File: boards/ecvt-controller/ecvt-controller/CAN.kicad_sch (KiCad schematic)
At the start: 12 parts, among them SW1 SW_SPST, SW2 SW_SPST, U1 TJA1051T-3

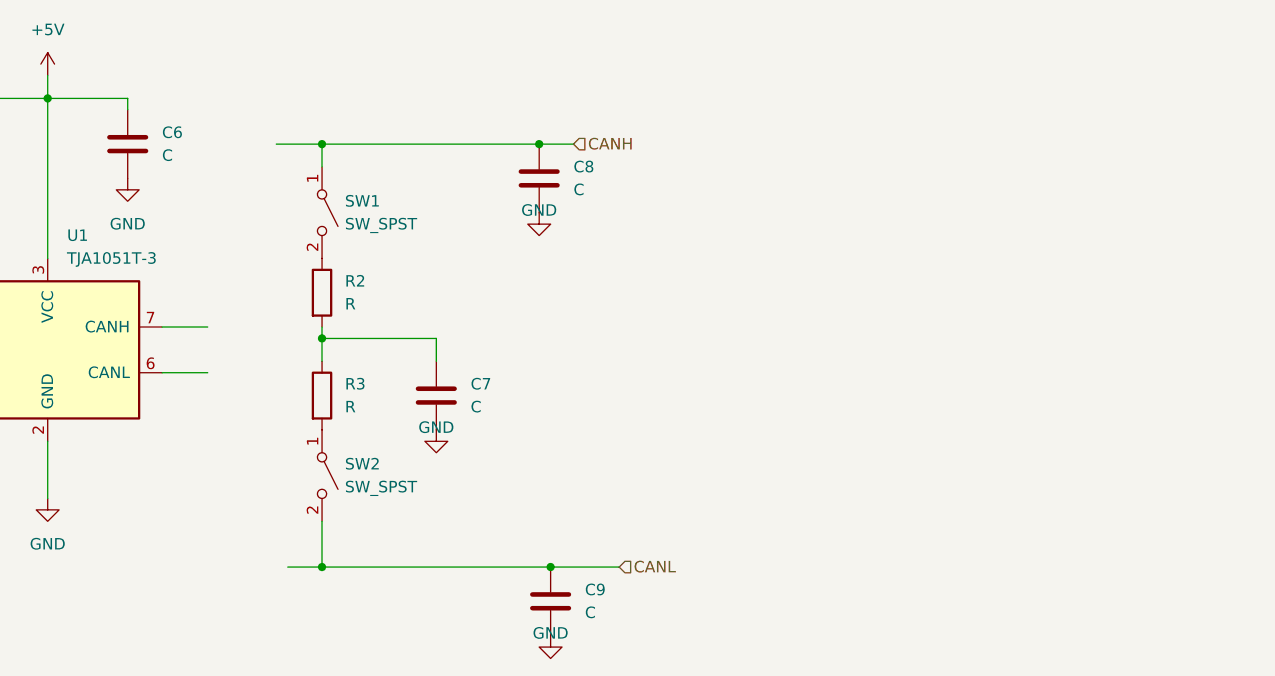
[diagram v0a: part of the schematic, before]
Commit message: CAN
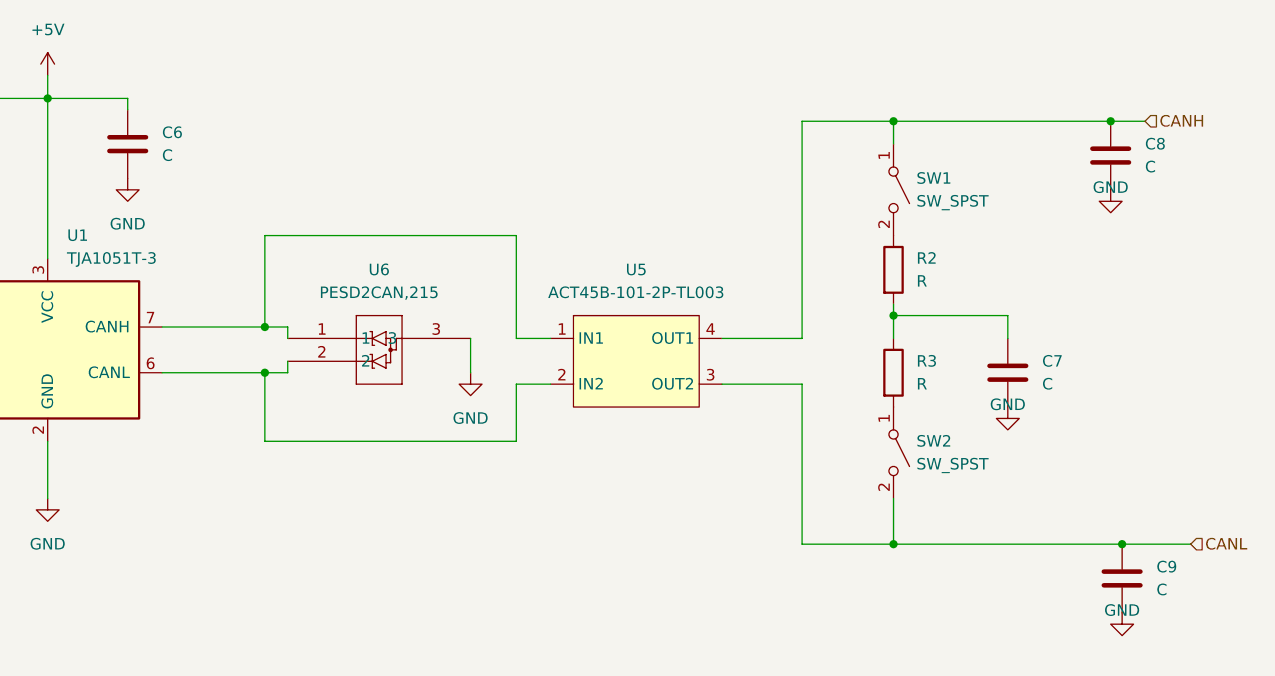
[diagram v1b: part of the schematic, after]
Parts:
- added U5: ACT45B-101-2P-TL003, baja_footprint_library:ACT45B-101-2P-TL003, symbol baja_symbol_library:ACT45B-101-2P-TL003
- added U6: PESD2CAN,215, Package_TO_SOT_SMD:SOT-23, symbol baja_symbol_library:ESD3V3AP-TP
- SW1, SW2: footprint (none) -> Button_Switch_THT:SW_DIP_SPSTx01_Slide_9.78x4.72mm_W7.62mm_P2.54mm
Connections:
- net CANH: now also U5.4 (OUT1)
- net CANL: now also U5.3 (OUT2)
- net GND: now also U6.3
- net at U1.6 (CANL): now also U5.2 (IN2), U6.2
- net at U1.7 (CANH): now also U5.1 (IN1), U6.1
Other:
- moved on the sheet: C7, C8, C9, R2, R3, SW1, SW2

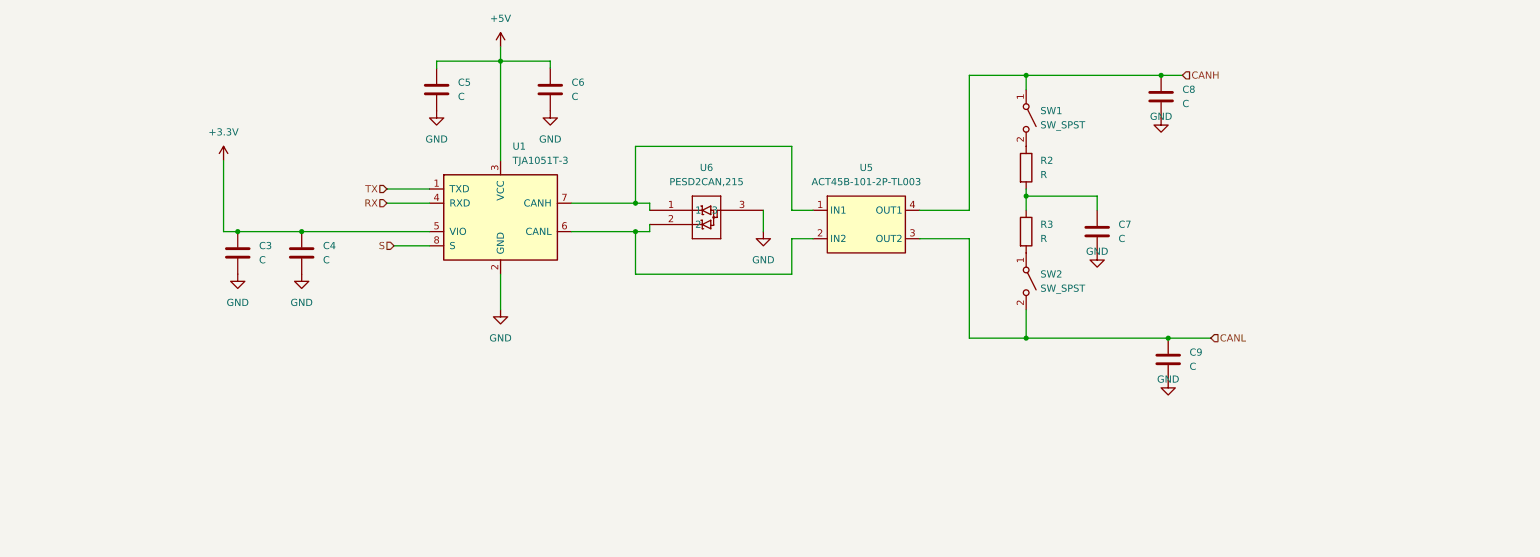
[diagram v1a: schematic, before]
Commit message: CAN actually done
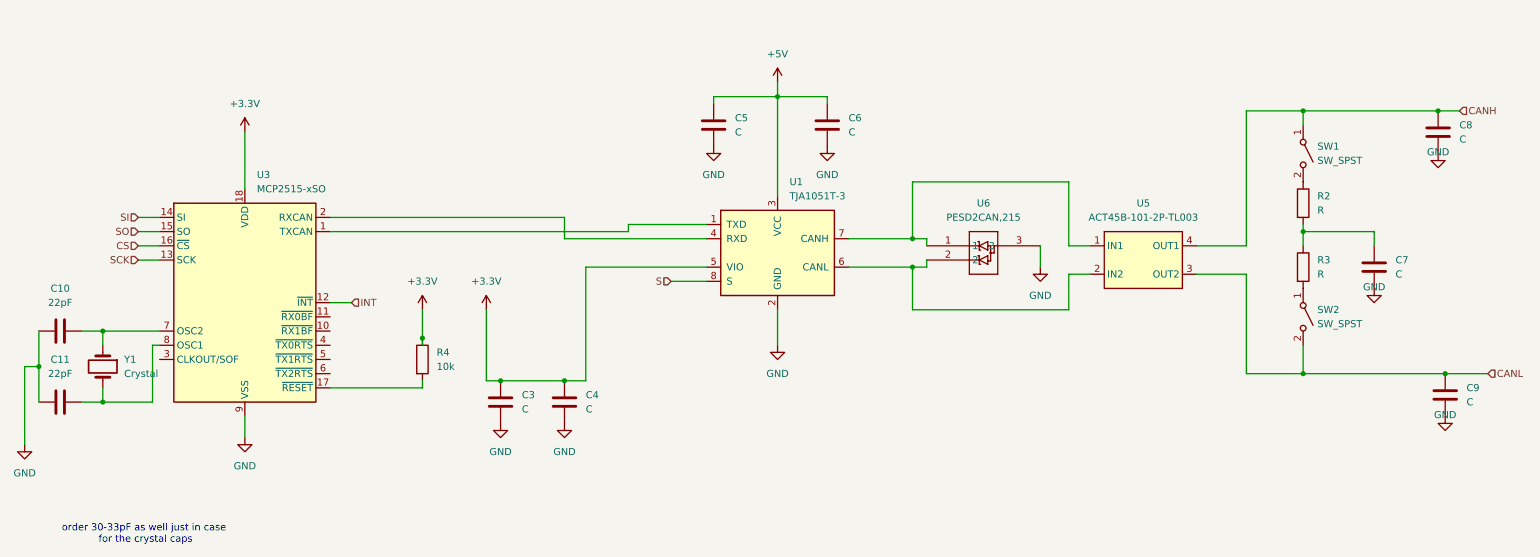
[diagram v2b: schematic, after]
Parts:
- added C10, C11: 22pF, symbol Device:C
- added R4: 10k, symbol Device:R
- added U3: MCP2515-xSO, Package_SO:SOIC-18W_7.5x11.6mm_P1.27mm, symbol Interface_CAN_LIN:MCP2515-xSO
- added Y1: Crystal, Crystal:Crystal_SMD_5032-2Pin_5.0x3.2mm_HandSoldering, symbol Device:Crystal
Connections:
- net +3.3V: now also R4.1, U3.18 (VDD)
- net GND: now also C10.1, C11.1, U3.9 (VSS)
- net RX: no longer names the net of U1.4 (RXD)
- net RX: now also U3.2 (RXCAN)
- net TX: no longer names the net of U1.1 (TXD)
- net TX: now also U3.1 (TXCAN)
- new net: R4.2, U3.17 (~{RESET})
- new net: C10.2, U3.7 (OSC2), Y1.1
- new net: C11.2, U3.8 (OSC1), Y1.2
- new net CS: U3.16 (~{CS})
- new net INT: U3.12 (~{INT})
- new net SCK: U3.13 (SCK)
- new net SI: U3.14 (SI)
- new net SO: U3.15 (SO)
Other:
- note added: "order 30-33pF as well just in case for the crystal caps"
- moved on the sheet: C3, C4, C5, C6, C7, C8, C9, R2, R3, SW1, SW2, U1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
